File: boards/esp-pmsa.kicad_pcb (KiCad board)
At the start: 2 copper layers, 40 x 47.5 mm, 12 parts, among them M1 PMSA003, U1 WeMos_D1_mini_Labels, U2 BME68x, U3 OPT3001DNPT

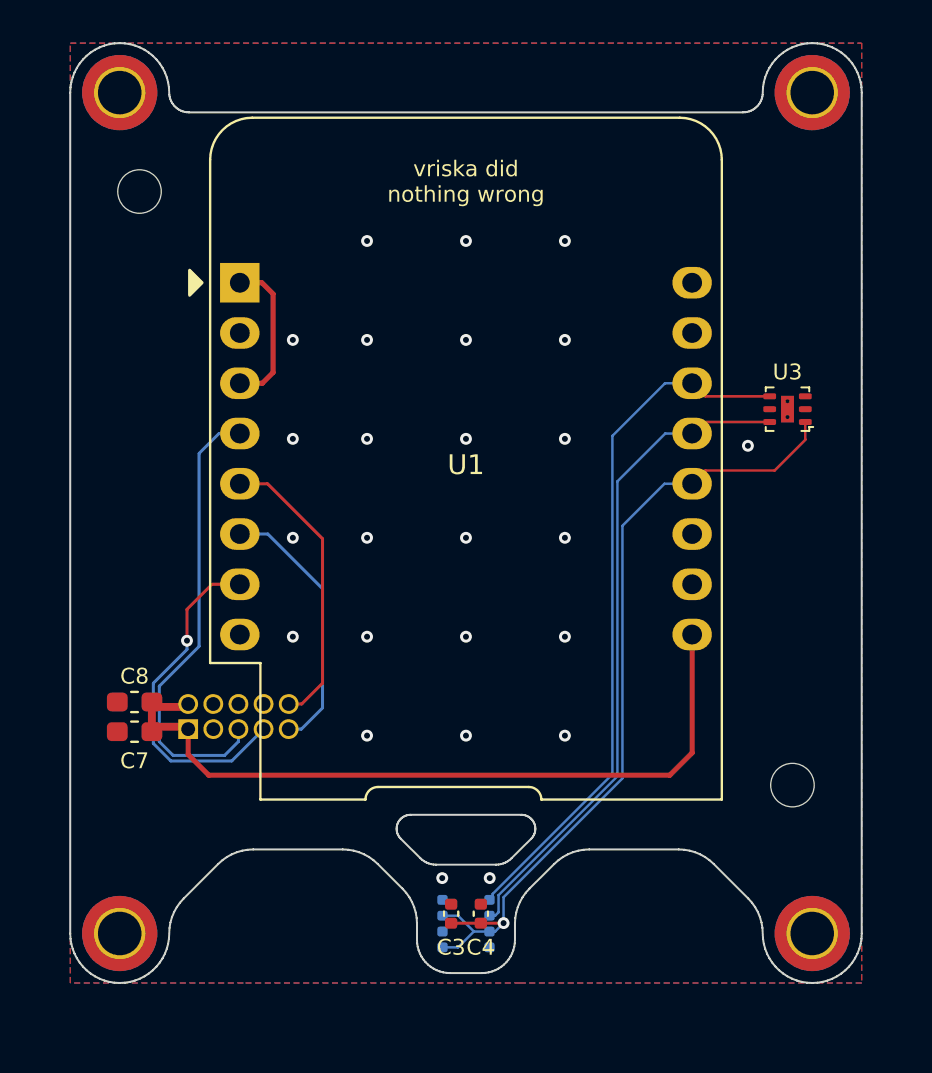
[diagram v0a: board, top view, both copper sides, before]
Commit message: Deploying to gh-pages from @ neg2led/esp-pmsa@e03a36f01e21f29b520752c6169685313d9a0f2f 🚀
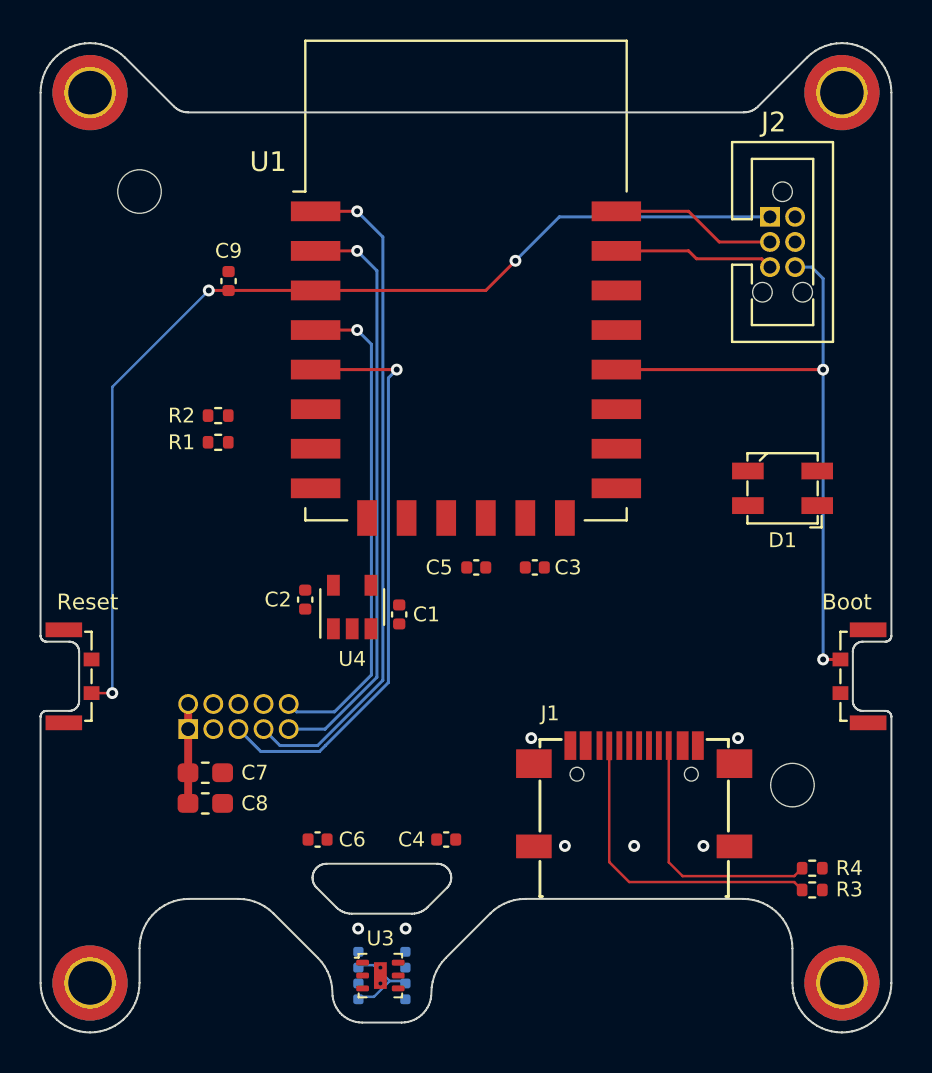
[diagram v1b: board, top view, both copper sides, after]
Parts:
- added C1: 10u, Capacitor_SMD:C_0402_1005Metric, F.Cu at (146.6, 103.9)
- added C2: 10u, Capacitor_SMD:C_0402_1005Metric, F.Cu at (141.9, 103.1)
- added C5: 1u, Capacitor_SMD:C_0402_1005Metric, F.Cu at (150.5, 101.5)
- added C6: 0.1u, Capacitor_SMD:C_0402_1005Metric, F.Cu at (142.5, 115.2)
- added C9: 0.1u, Capacitor_SMD:C_0402_1005Metric, F.Cu at (138.0, 87.0)
- added D1: APA104-12-3535, 21-SnapEDA-zip:LED_APA104-12-3535, F.Cu at (166.0, 97.5)
- added J1: USB_C_Receptacle_USB2.0_304S-ACP16, 41-EasyEDA-Edits:USB-C-SMD_TYPEC-304S-ACP16, F.Cu at (158.5, 113.0)
- added J2: ESP-PROG, 11-My-Edits:TC2030_IDCBox_2x03_P1.25mm_Vertical_3D, F.Cu at (166.0, 85.0)
- added R1: 4k7, Resistor_SMD:R_0402_1005Metric, F.Cu at (137.5, 95.2)
- added R2: 4k7, Resistor_SMD:R_0402_1005Metric, F.Cu at (137.5, 93.8)
- added R3: 5k1, Resistor_SMD:R_0402_1005Metric, F.Cu at (167.5, 117.8)
- added R4: 5k1, Resistor_SMD:R_0402_1005Metric, F.Cu at (167.5, 116.7)
- added SW1: Reset, 41-EasyEDA-Edits:SW-SMD_SKSLLAE010-3D, F.Cu at (130.4, 107.0)
- added SW2: Boot, 41-EasyEDA-Edits:SW-SMD_SKSLLAE010-3D, F.Cu at (169.6, 107.0)
- added U4: XC6220B331MR, Package_TO_SOT_SMD:SOT-23-5, F.Cu at (144.2, 103.5)
- C3: value 1uF -> 1u
- C4: value 100nF -> 0.1u
- C7, C8: value 10uF -> 10u
- U1: value WeMos_D1_mini_Labels -> ESP32-C3F; footprint 11-My-Edits:WEMOS_D1_mini -> 11-My-Edits:ESP-12H
- moved U3 35.3 mm to (145.7, 122.1), turned to 0 degrees
- moved C3 18.0 mm to (153.5, 101.5), turned to 0 degrees
- moved U1 9.00 mm to (150.0, 87.0)
- moved C8 6.25 mm to (136.8, 113.4), turned to 0 degrees
- moved U2 5.00 mm to (145.8, 122.1)
- moved C4 4.14 mm to (149.0, 115.2), turned to 180 degrees
- moved C7 4.13 mm to (136.8, 111.9), turned to 0 degrees
- moved H2 2.92 mm to (169.0, 122.5)
- moved H4 2.92 mm to (131.0, 122.5)
- moved H1 1.50 mm to (131.0, 77.5)
- moved H3 1.50 mm to (169.0, 77.5)
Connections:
- C3 pad 1: Board_1-/VCC_SENS -> Board_1-/VCC_BME
- C4 pad 1: Board_1-GND -> Board_1-/VCC_BME
- C4 pad 2: Board_1-/VCC_SENS -> Board_1-GND
- M1 pad 8: Board_1-Net-(M1-Pad8) -> Board_1-Net-(M1-Pad6)
- U1 pad 1: Board_1-/~WAKE -> Board_1-/PMS_RX
- U1 pad 10: Board_1-GND -> Board_1-Net-(U1-Pad10)
- U1 pad 11: Board_1-Net-(U1-Pad11) -> Board_1-Net-(U1-Pad10)
- U1 pad 12: Board_1-/VCC_SENS -> Board_1-/VCC_ALS
- U1 pad 13: Board_1-/SDA -> Board_1-/VCC_BME
- U1 pad 14: Board_1-/SCL -> Board_1-Net-(U1-Pad10)
- U1 pad 15: Board_1-/U0RXD -> Board_1-GND
- U1 pad 16: Board_1-/U0TXD -> (no net)
- U1 pad 2: Board_1-Net-(U1-Pad2) -> Board_1-/PMS_TX
- U1 pad 3: Board_1-/~WAKE -> Board_1-/~RST
- U1 pad 4: Board_1-/~PMS_RST -> Board_1-/~PMS_SET
- U1 pad 5: Board_1-/~PMS_SET -> Board_1-/~PMS_RST
- U1 pad 6: Board_1-/PMS_TX -> Board_1-/SDA
- U1 pad 7: Board_1-/PMS_RX -> Board_1-/SCL
- U1 pad 9: Board_1-+5V -> Board_1-Net-(U1-Pad10)
- U2 pad 2: Board_1-/VCC_SENS -> Board_1-/VCC_BME
- U2 pad 6: Board_1-/VCC_SENS -> Board_1-/VCC_BME
- U2 pad 8: Board_1-/VCC_SENS -> Board_1-/VCC_BME
- U3 pad 1: Board_1-/VCC_SENS -> Board_1-/VCC_ALS
- U3 pad 5: Board_1-Net-(U3-Pad5) -> (no net)
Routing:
- net Board_1-/~RST: track 0.00 -> 53.6 mm, vias 0 -> 3
- net Board_1-/VCC_SENS: track 42.8 -> 0.00 mm, vias 1 -> 0
- net Board_1-/SCL: track 35.5 -> 0.00 mm
- net Board_1-+5V: track 39.4 -> 5.03 mm
- net Board_1-/SDA: track 33.8 -> 0.00 mm
- net Board_1-/~BOOT: track 0.00 -> 32.2 mm, vias 0 -> 2
- net Board_1-/PMS_RX: track 17.0 -> 34.1 mm
- net Board_1-Net-(J1-PadA5): track 0.00 -> 16.2 mm
- net Board_1-/PMS_TX: track 13.5 -> 29.6 mm, vias 0 -> 1
- net Board_1-Net-(J1-PadB5): track 0.00 -> 13.1 mm
- net Board_1-/~PMS_SET: track 14.8 -> 25.0 mm, vias 0 -> 1
- net Board_1-/U0TXD: track 0.00 -> 8.41 mm
- net Board_1-/U0RXD: track 0.00 -> 8.10 mm
- net Board_1-/~WAKE: track 7.79 -> 0.00 mm
- net Board_1-/~PMS_RST: track 23.1 -> 29.6 mm, vias 0 -> 1
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- removed copper zone on B.Cu, net Board_1-GND
- removed copper zone on F.Cu, net Board_1-GND
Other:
- board size 40 x 47.5 mm -> 43 x 50 mm
- board text added: "Boot"
- board text added: "Reset"
- board text removed: "vriska did nothing wrong"
